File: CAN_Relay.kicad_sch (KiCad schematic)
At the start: 41 parts, among them J1 430450601, J4 691305340008, J5 691305340008, U1 Teensy4.0, U2 BTS716GB, U3 BTS716GB, U4 ADM3057EBRWZ, U5 LM22676MRE-5.0/NOPB

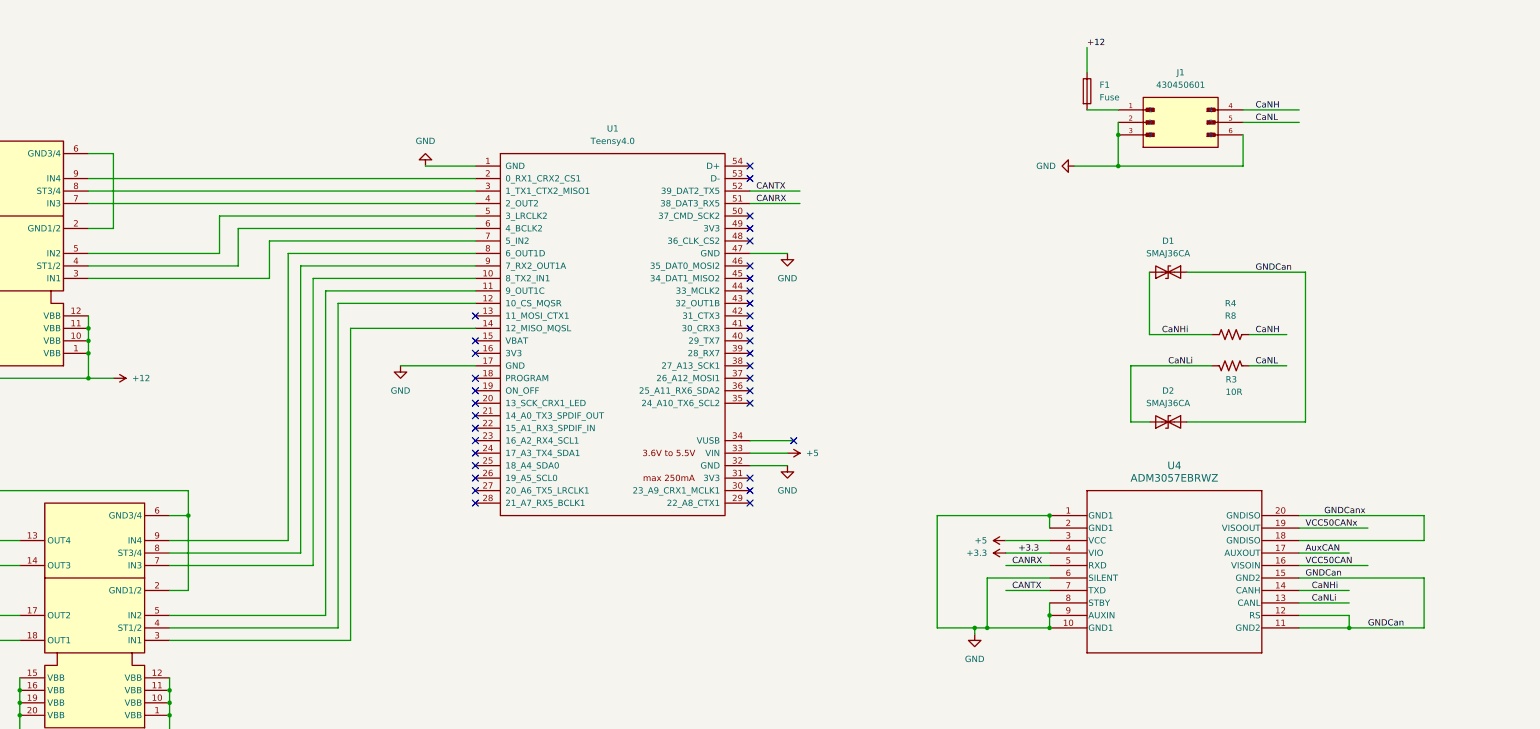
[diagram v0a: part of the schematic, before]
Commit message: added smd pins for teensy
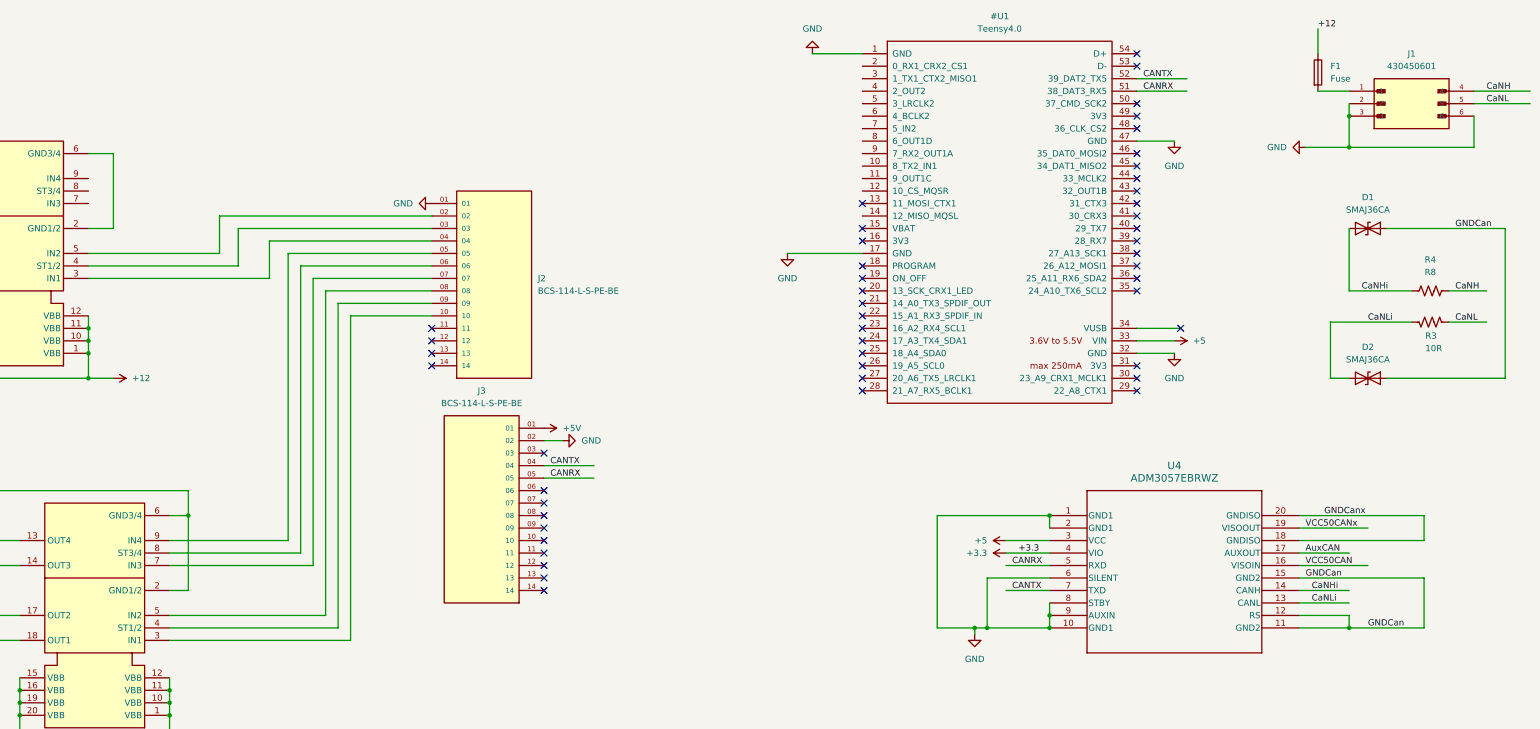
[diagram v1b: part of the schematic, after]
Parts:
- added J2, J3: BCS-114-L-S-PE-BE, BCS:SAMTEC_BCS-114-L-S-PE-BE, symbol BCS-114-L-S-PE-BE:BCS-114-L-S-PE-BE
- renumbered U1 to #U1
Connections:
- net CANRX: now also J3.05
- net CANTX: now also J3.04
- net GND: now also J2.01, J3.02
- net at U3.3 (IN1): now also J2.10; no longer #U1.14 (12_MISO_MQSL)
- net at U3.4 (ST1/2): now also J2.09; no longer #U1.12 (10_CS_MQSR)
- net at U3.5 (IN2): now also J2.08; no longer #U1.11 (9_OUT1C)
- net at U3.7 (IN3): now also J2.07; no longer #U1.10 (8_TX2_IN1)
- net at U3.8 (ST3/4): now also J2.06; no longer #U1.9 (7_RX2_OUT1A)
- net at U3.9 (IN4): now also J2.05; no longer #U1.8 (6_OUT1D)
- net at U2.3 (IN1): now also J2.04; no longer #U1.7 (5_IN2)
- net at U2.4 (ST1/2): now also J2.03; no longer #U1.6 (4_BCLK2)
- net at U2.5 (IN2): now also J2.02; no longer #U1.5 (3_LRCLK2)
- net at U2.7 (IN3): no longer #U1.4 (2_OUT2)
- net at U2.8 (ST3/4): no longer #U1.3 (1_TX1_CTX2_MISO1)
- net at U2.9 (IN4): no longer #U1.2 (0_RX1_CRX2_CS1)
- new net +5V: J3.01
- no-connect marks 36 -> 50
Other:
- moved on the sheet: D1, D2, F1, J1, R3, R4
